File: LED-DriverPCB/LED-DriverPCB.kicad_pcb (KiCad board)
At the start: 4 copper layers, 246 x 144.3 mm, 51 parts, among them J1 Screw_Terminal_01x03, J12 Screw_Terminal_01x02, J13 Screw_Terminal_01x02, J14 Screw_Terminal_01x02, J15 Screw_Terminal_01x02, J16 Screw_Terminal_01x02, J17 Screw_Terminal_01x02, J18 Screw_Terminal_01x02, J19 Screw_Terminal_01x02, J2 Screw_Terminal_01x03, J20 Conn_ARM_SWD_TagConnect_TC2030, J3 Screw_Terminal_01x03, J4 Screw_Terminal_01x03, J5 Screw_Terminal_01x03, J6 Screw_Terminal_01x03, J7 Screw_Terminal_01x03, J8 Screw_Terminal_01x03, J9 USB_C_Receptacle_USB2.0_16P, U1 STM32F103RCTx, U2 TXB0108PW, U3 AMS1117-3.3, U4 USBLC6-2SC6, X1 8MHz

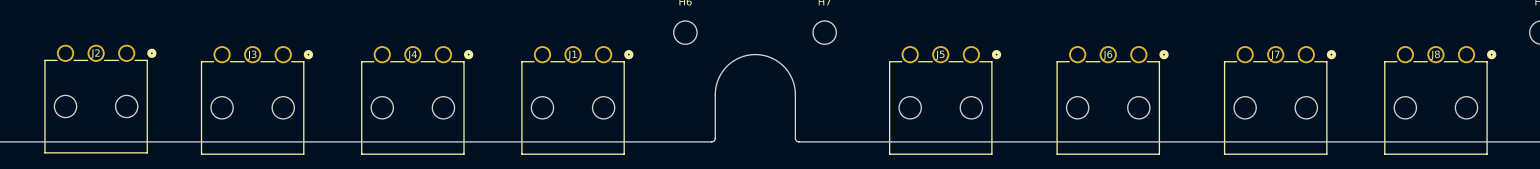
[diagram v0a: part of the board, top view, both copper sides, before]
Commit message: Aligned connectors
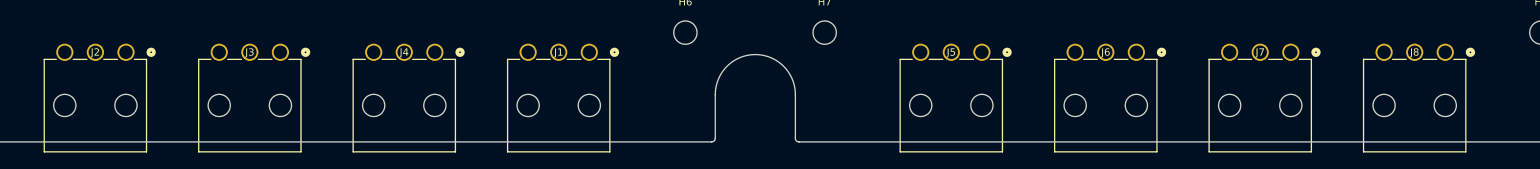
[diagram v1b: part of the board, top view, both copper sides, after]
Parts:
- moved J8 2.93 mm to (323.3, 203.0)
- moved J7 2.15 mm to (302.1, 203.0)
- moved J1 1.99 mm to (205.7, 203.0)
- moved J5 1.49 mm to (259.6, 203.0)
- moved J4 1.22 mm to (184.5, 203.0)
- moved J3 0.51 mm to (163.3, 203.0)
- moved J6 0.47 mm to (280.9, 203.0)
- moved J2 0.17 mm to (142.1, 203.0)
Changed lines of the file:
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@@
 	(footprint "39303037:CONN_5569-03A4&slash_5_MOL"
 		(layer "F.Cu")
-		(at 163.695599 203.3229)
+		(at 163.307099 203)
 		(tags "39303037 ")
 		(property "Reference" "J3"
@@
 	(footprint "39303037:CONN_5569-03A4&slash_5_MOL"
 		(layer "F.Cu")
-		(at 281.195599 203.3229)
+		(at 280.856599 203)
 		(tags "39303037 ")
 		(property "Reference" "J6"
@@
 	(footprint "39303037:CONN_5569-03A4&slash_5_MOL"
 		(layer "F.Cu")
-		(at 142.195599 203.1409)
+		(at 142.096099 203)
 		(tags "39303037 ")
 		(property "Reference" "J2"
@@
 	(footprint "39303037:CONN_5569-03A4&slash_5_MOL"
 		(layer "F.Cu")
-		(at 304.195599 203.3229)
+		(at 302.067599 203)
 		(tags "39303037 ")
 		(property "Reference" "J7"
@@
 	(footprint "39303037:CONN_5569-03A4&slash_5_MOL"
 		(layer "F.Cu")
-		(at 326.195599 203.3229)
+		(at 323.278599 203)
 		(tags "39303037 ")
 		(property "Reference" "J8"
@@
 	(footprint "39303037:CONN_5569-03A4&slash_5_MOL"
 		(layer "F.Cu")
-		(at 185.695599 203.3229)
+		(at 184.518099 203)
 		(tags "39303037 ")
 		(property "Reference" "J4"
@@
 	(footprint "39303037:CONN_5569-03A4&slash_5_MOL"
 		(layer "F.Cu")
-		(at 207.695599 203.3229)
+		(at 205.729099 203)
 		(tags "39303037 ")
 		(property "Reference" "J1"
@@
 	(footprint "39303037:CONN_5569-03A4&slash_5_MOL"
 		(layer "F.Cu")
-		(at 258.195599 203.3229)
+		(at 259.645599 203)
 		(tags "39303037 ")
 		(property "Reference" "J5"
